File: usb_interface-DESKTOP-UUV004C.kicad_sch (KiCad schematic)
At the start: 13 parts, among them J2 USB_B_Micro, U4 FT234XD-R

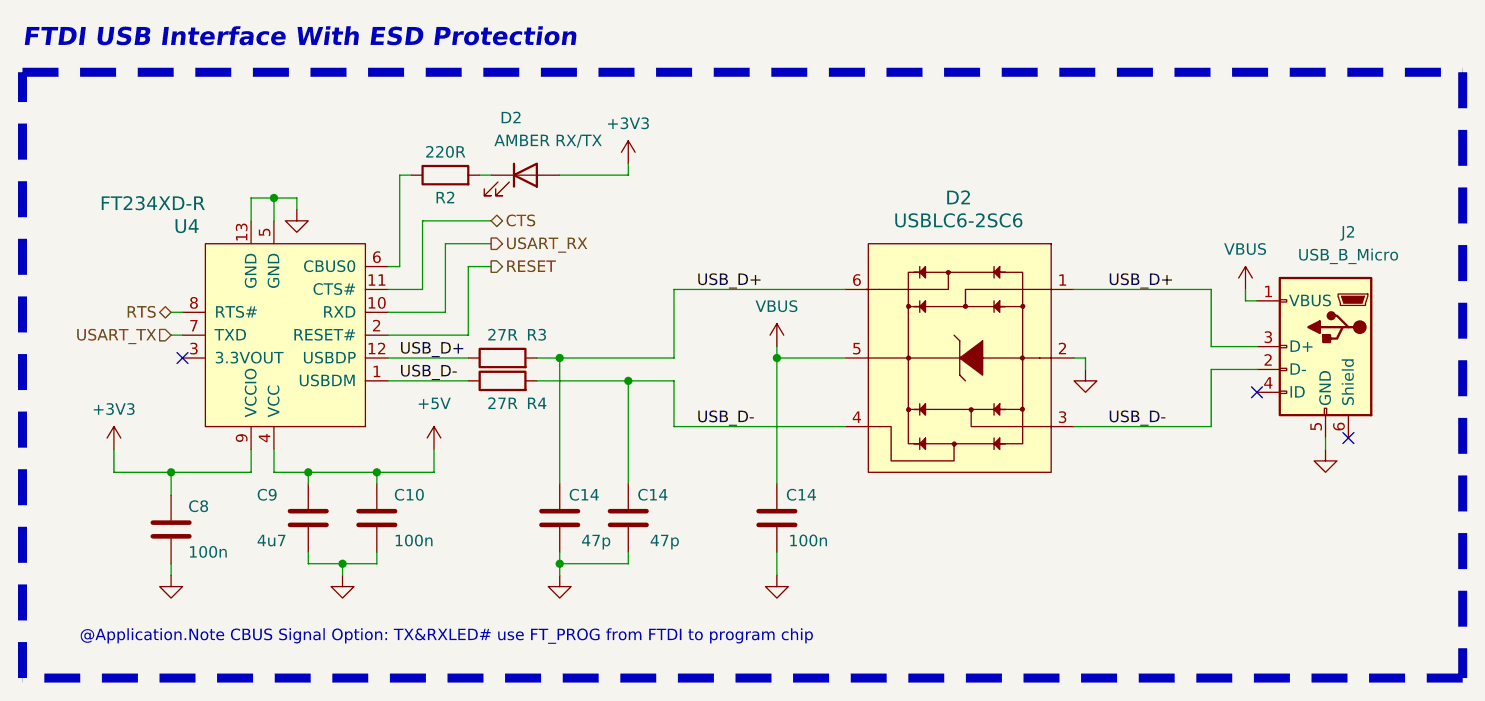
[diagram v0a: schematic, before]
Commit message: Done power
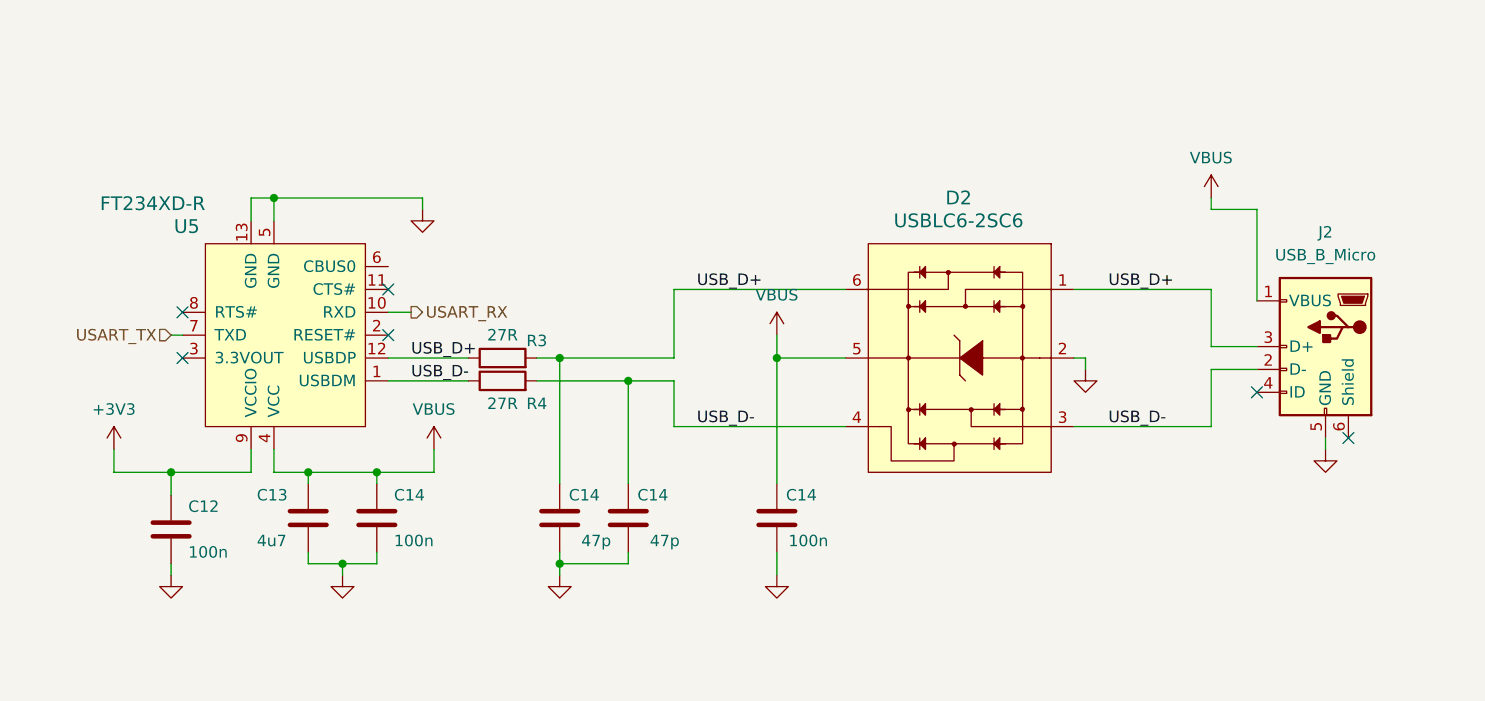
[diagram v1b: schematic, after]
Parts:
- removed D2: AMBER RX/TX, LED_SMD:LED_0603_1608Metric, symbol Device:LED
- removed R2: 220R, Resistor_SMD:R_0402_1005Metric, symbol Device:R
- D2: JLC # C7519 -> (none)
- J2: footprint Connector_USB:USB_Micro-B_Amphenol_10103594-0001LF_Horizontal -> footprints:AMPHENOL_10103593-0001LF
- U5: renamed from U4; JLC # C132158 -> (none)
- renumbered C8 to C12, C9 to C13, C10 to C14
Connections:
- net +5V is gone; now on net VBUS: C13.1, C14.1, U5.4 (VCC)
- net CTS: no longer names the net of U5.11 (CTS#)
- net RESET: no longer names the net of U5.2 (RESET#)
- net RTS: no longer names the net of U5.8 (RTS#)
- no-connect marks 3 -> 6
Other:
- note removed: "@Application.Note CBUS Signal Option: TX&RXLED# use FT_PROG from FTDI to program chip"
- note removed: "FTDI USB Interface With ESD Protection"
